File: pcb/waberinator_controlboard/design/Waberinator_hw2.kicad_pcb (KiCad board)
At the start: 2 copper layers, 50.5 x 99.5 mm, 119 parts, among them J1 Conn_01x04_Pin, J17 GX16-4, J18 GX12-4, J19 GX12-4, J20 GX12-4, J21 GX12-4, J22 GX12-4, J23 GX12-4, J24 GX12-4, J25 GX12-4, J26 GX12-4, J27 Conn_01x04, J28 Conn_01x04, J29 Conn_01x04, J4 Conn_01x08_Pin, Q1 AOSP21321, Q2 SISHA04DN-T1-GE3, Q3 SISHA04DN-T1-GE3, Q4 SISHA04DN-T1-GE3, Q5 SISHA04DN-T1-GE3, Q6 SISHA04DN-T1-GE3, Q7 SISHA04DN-T1-GE3, SW1 SW_SPDT, U1 STM32F030R8Tx, U2 AMS1117-3.3, U3 LM73606QRNPRQ1, U4 LM75B, U5 MCP14A0304xMNY, U6 MCP14A0304xMNY, U7 MCP14A0304xMNY

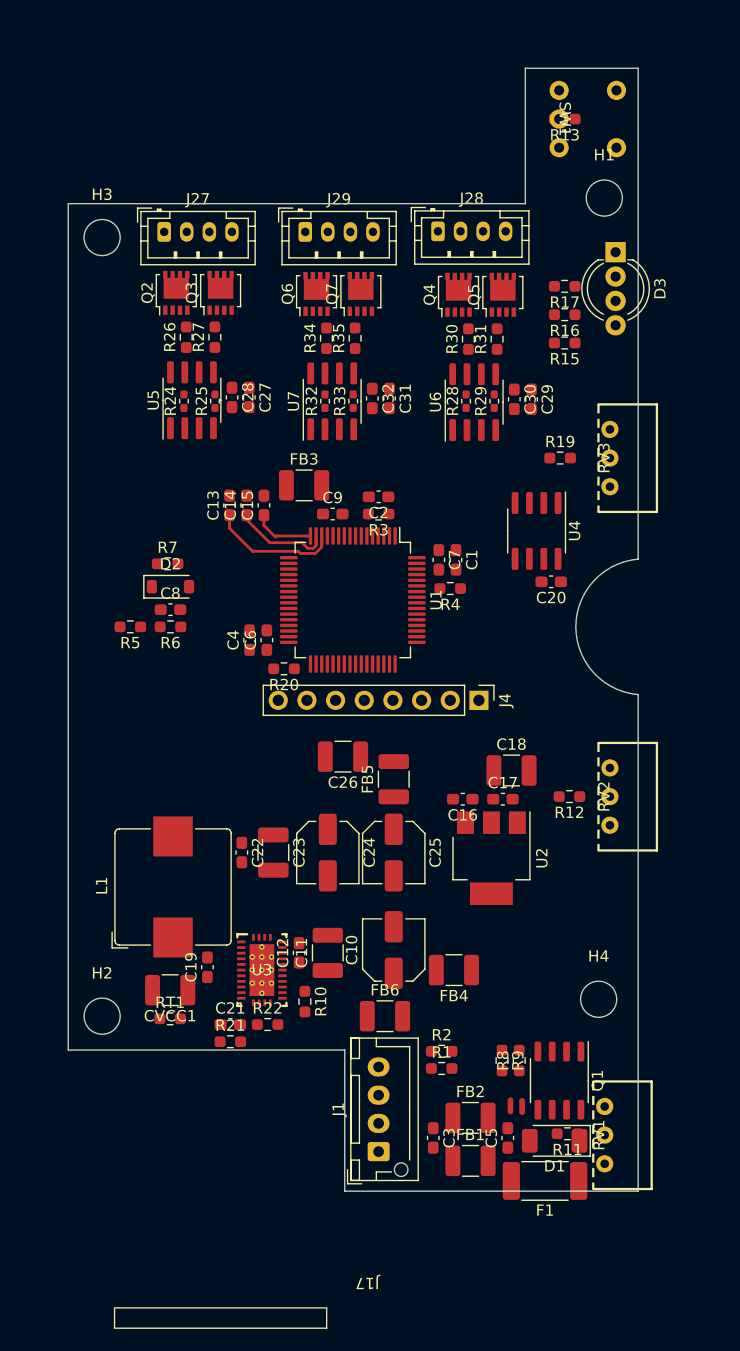
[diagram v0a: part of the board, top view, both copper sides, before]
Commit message: finalize BOL
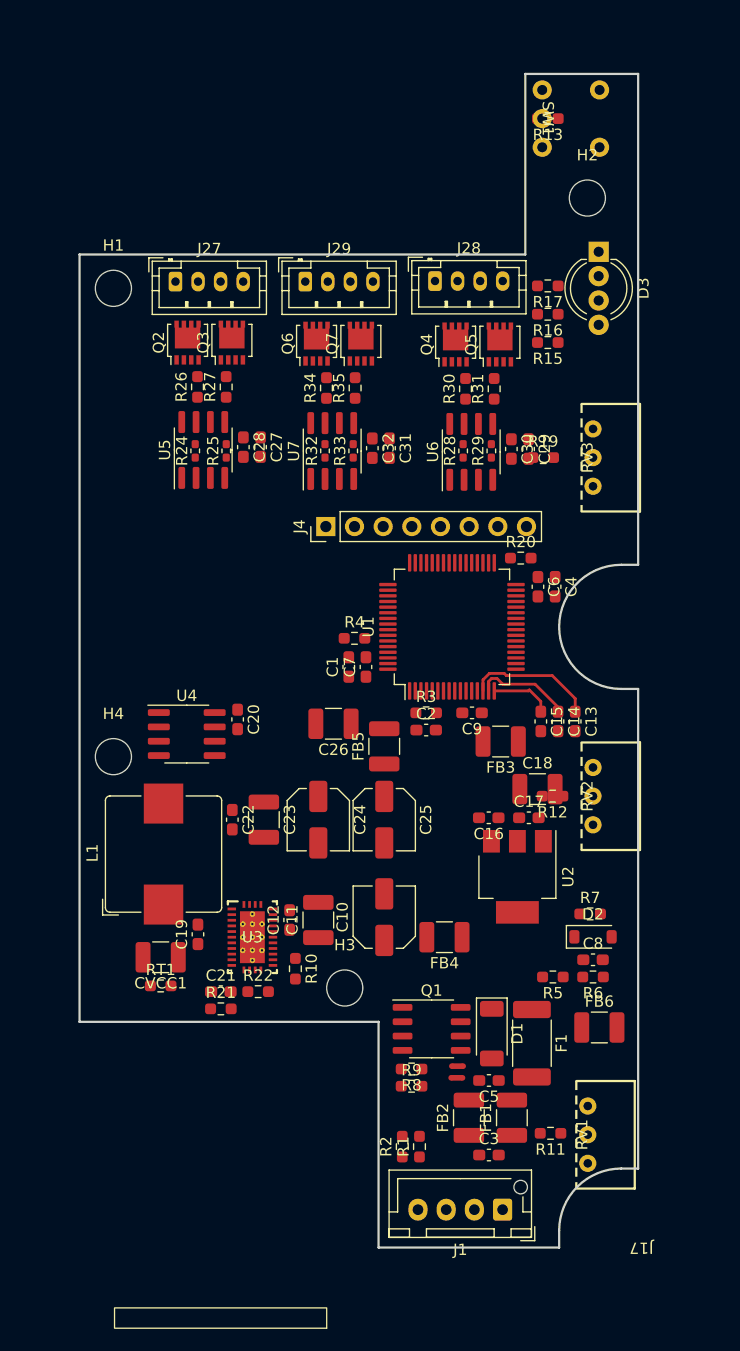
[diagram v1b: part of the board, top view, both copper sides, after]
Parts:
- moved H2 84.3 mm to (111.5, 134.5)
- moved H3 69.9 mm to (90.0, 204.5)
- moved C8 48.6 mm to (112.0, 202.0)
- moved D2 48.6 mm to (112.0, 200.0)
- moved R5 48.6 mm to (108.4, 203.5)
- moved R6 48.6 mm to (112.0, 203.5)
- moved R7 48.6 mm to (111.7, 197.9)
- moved H4 48.1 mm to (69.5, 184.0)
- moved H1 44.2 mm to (69.5, 142.5)
- moved C13 36.1 mm to (110.4, 180.9), turned to -90 degrees
- moved U4 35.8 mm to (76.0, 182.0), turned to 0 degrees
- moved C14 33.6 mm to (108.9, 180.9), turned to -90 degrees
- moved C15 31.1 mm to (107.4, 180.9), turned to -90 degrees
- moved C20 30.3 mm to (80.5, 180.7), turned to -90 degrees
- moved FB3 28.6 mm to (103.8, 182.7), turned to 180 degrees
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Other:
- board size 50.5 x 99.5 mm -> 49.5 x 104 mm
